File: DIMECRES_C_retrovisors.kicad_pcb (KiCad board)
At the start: 2 copper layers, 108.3 x 91.8 mm, 100 parts, among them J10 Vbat, J2 DE9_Pins, J3 Conn_01x05_Pin, J4 Motor3, J5 DE9_Pins, J6 Intermitente, J7 Calentador, J8 Motor2, J9 Motor1, Q1 DTC144E, Q2 DTC144E, Q3 DTC144E, SW1 SW_DPDT_G6S, SW10 SW_Push, SW2 UN/FOLD, SW3 HEAT, SW4 UP, SW5 DOWN, SW6 LEFT, SW7 RIGHT, SW8 FN01B, SW9 FN01B, U1 CH201, U10 LM1117DT-5.0, U2 ADM7160, U3 LM2596S-ADJ, U4 L298N, U5 MCP2551-I-SN, U6 ADA4511-2, U7 PIC18F4480-IP, U8 LSF0002, Y1 Crystal

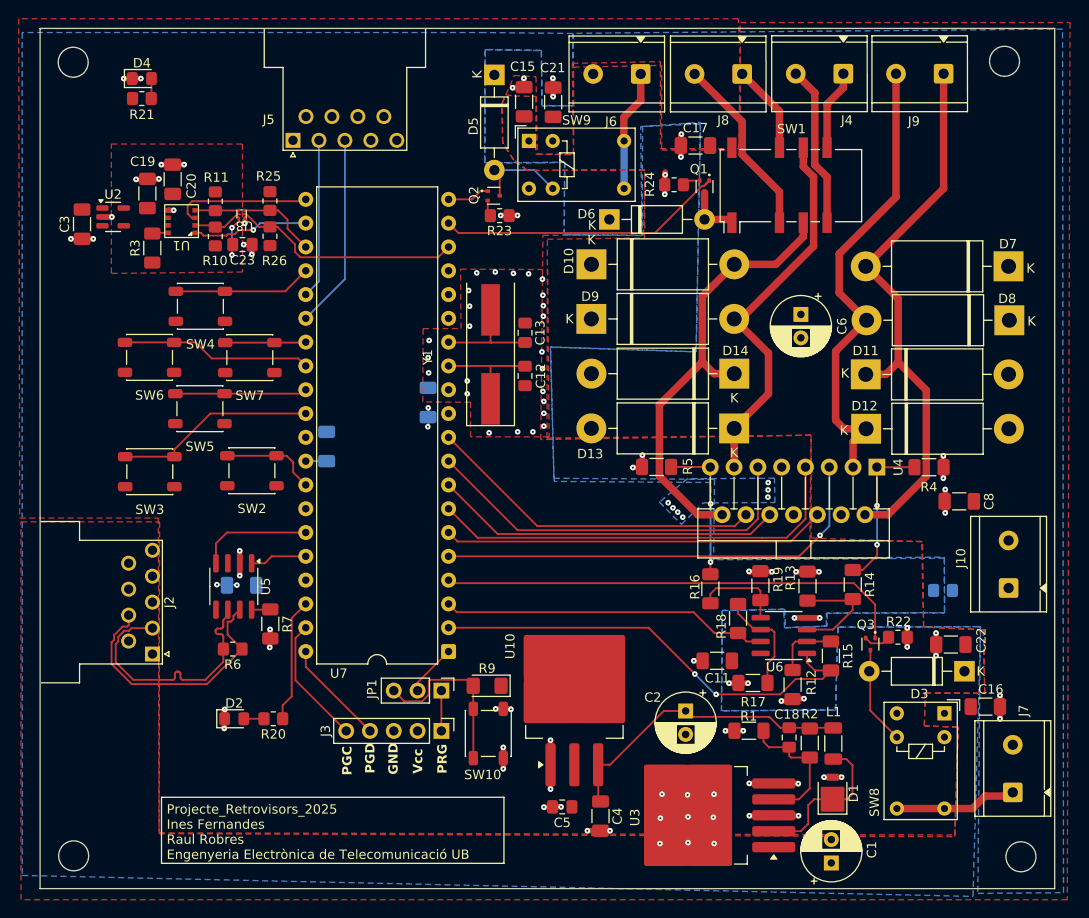
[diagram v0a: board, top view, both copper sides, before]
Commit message: .,.
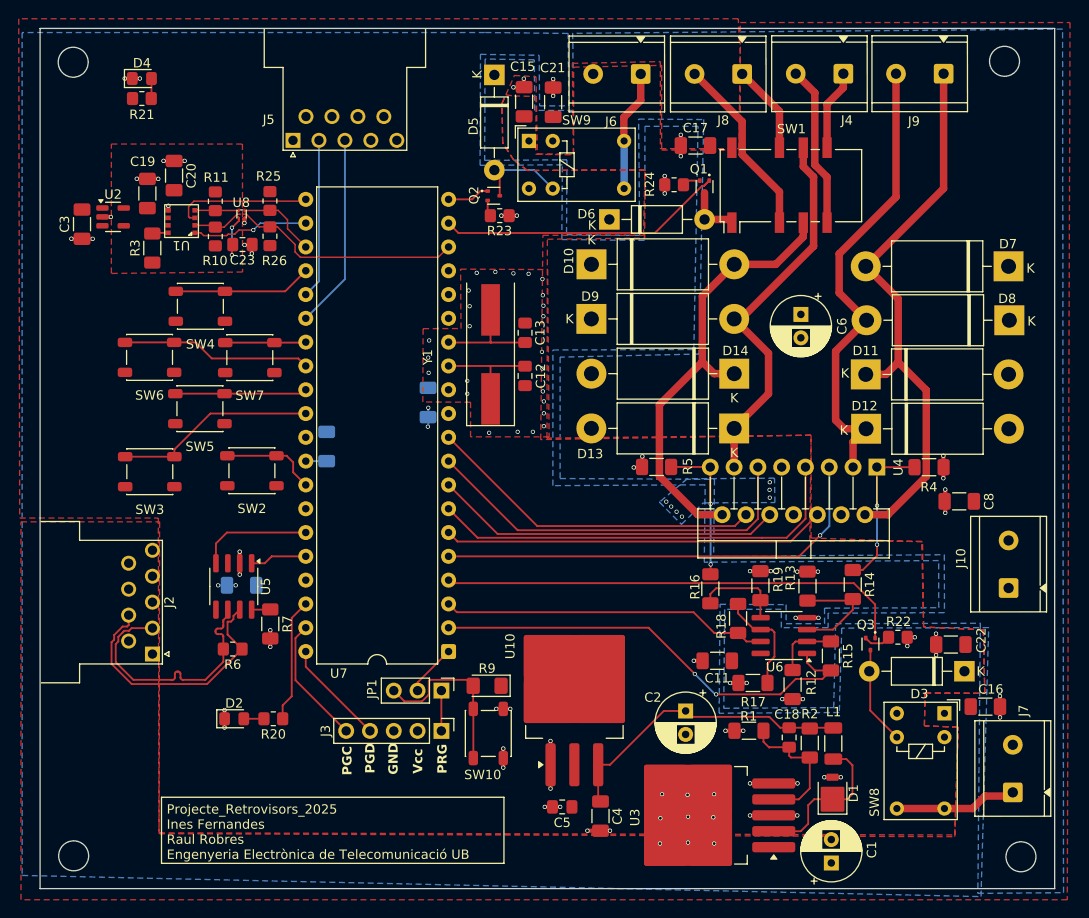
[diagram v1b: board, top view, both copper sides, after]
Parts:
- removed R8: 0, Resistor_SMD:R_0805_2012Metric_Pad1.20x1.40mm_HandSolder
- moved C20 0.42 mm to (100.8, 64.7)
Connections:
- net Net-(D1-K) renamed /OUT_BUCK
- net Net-(D3-A) renamed /Tran_Cal
- net Net-(D5-A) renamed /Tran_Int
- net Net-(U1-SCL) renamed /SCL1
- net Net-(U1-SDA) renamed /SDA1
- net Net-(U3-FB) renamed /FB
- net Net-(U6A-+) renamed /OPA_P
- net Net-(U6A--) renamed /OPA_N
- net Net-(U6B-+) renamed /OPB_P
- net Net-(U6B--) renamed /OPB_N
- net Net-(U7-OSC1/CLKI/RA7) renamed /OSC1
- net Net-(U7-OSC2/CLKO/RA6) renamed /OSC2
- C15 pad 2: GNDPWR -> GND
- C16 pad 2: GNDPWR -> GND
- C6 pad 2: GNDPWR -> GND
- C8 pad 2: GNDPWR -> GND
- D11 pad 2: GNDPWR -> GND
- D12 pad 2: GNDPWR -> GND
- D13 pad 2: GNDPWR -> GND
- D14 pad 2: GNDPWR -> GND
- J10 pad 2: GNDPWR -> GND
- J6 pad 2: GNDPWR -> GND
- J7 pad 2: GNDPWR -> GND
- R12 pad 1: GNDPWR -> GND
- R17 pad 1: GNDPWR -> GND
- R4 pad 2: GNDPWR -> GND
- R5 pad 2: GNDPWR -> GND
- U4 pad 8: GNDPWR -> GND
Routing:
- net GNDPWR: track 17.1 -> 0.00 mm, vias 14 -> 0
- net GND: track 69.1 -> 80.6 mm, vias 90 -> 104
- removed copper zone on B.Cu, net GNDPWR
